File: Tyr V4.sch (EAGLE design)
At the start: 190 parts, among them J1 TYR_TYR_DISPLAY, U1 TYR_ATMEGA32U4, U2 CONTROLLER_PRTR5V0U2X, U4 TYR_TPS2552, X1 CONTROLLER_USB-C-12PUSB-C-12P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, Y1 16Mhz

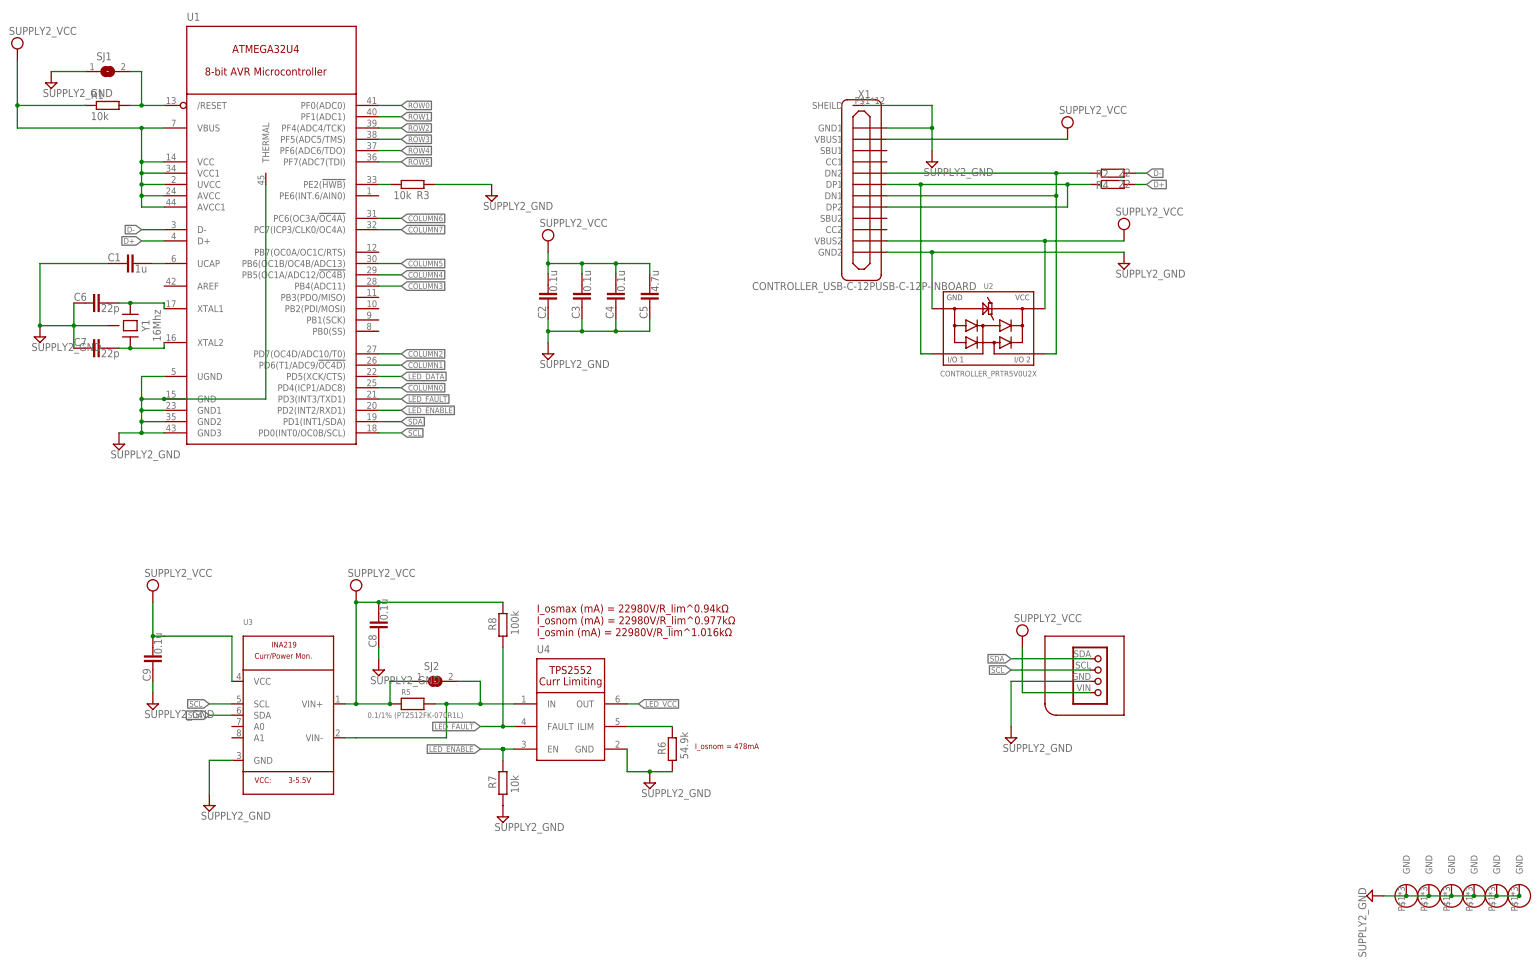
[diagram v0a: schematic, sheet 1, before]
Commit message: Update pads
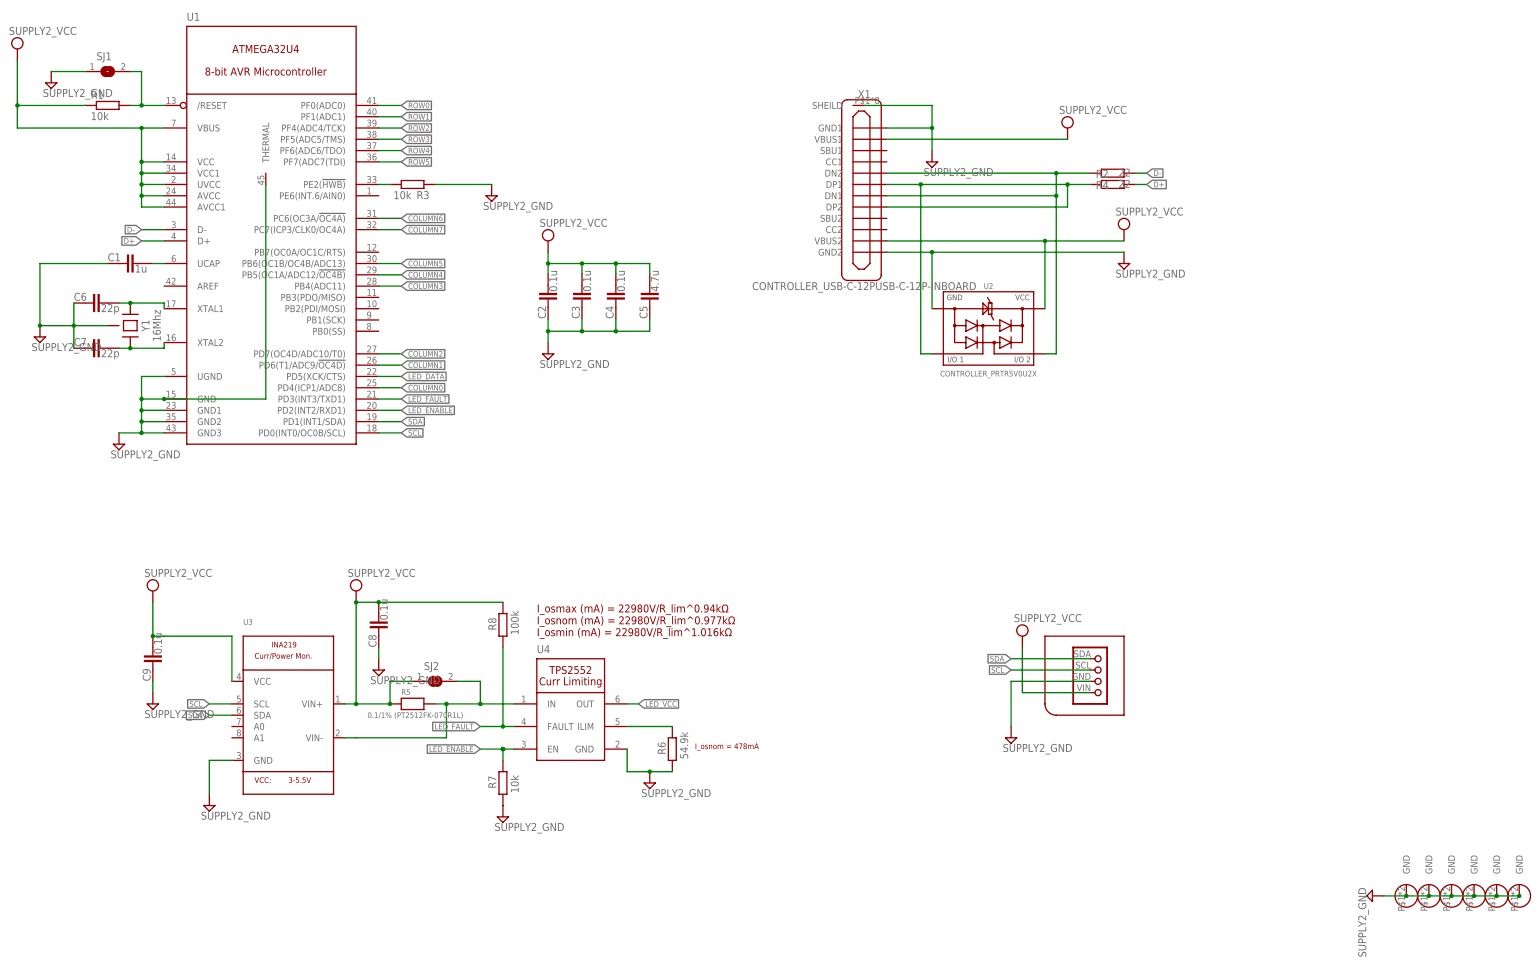
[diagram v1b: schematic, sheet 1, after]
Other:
- moved on the sheet: X1
